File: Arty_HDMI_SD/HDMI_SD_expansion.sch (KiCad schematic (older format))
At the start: 47 parts, among them J1 0015912120, J2 1140084168, J3 0015912120, J4 2000-1-2-41-00-BK, J5 UE27AC54100, J6 0015912120, U1 TPS61232DRCT, U2 MAX3421EEHJ, Y1 KX-7_12,MHz

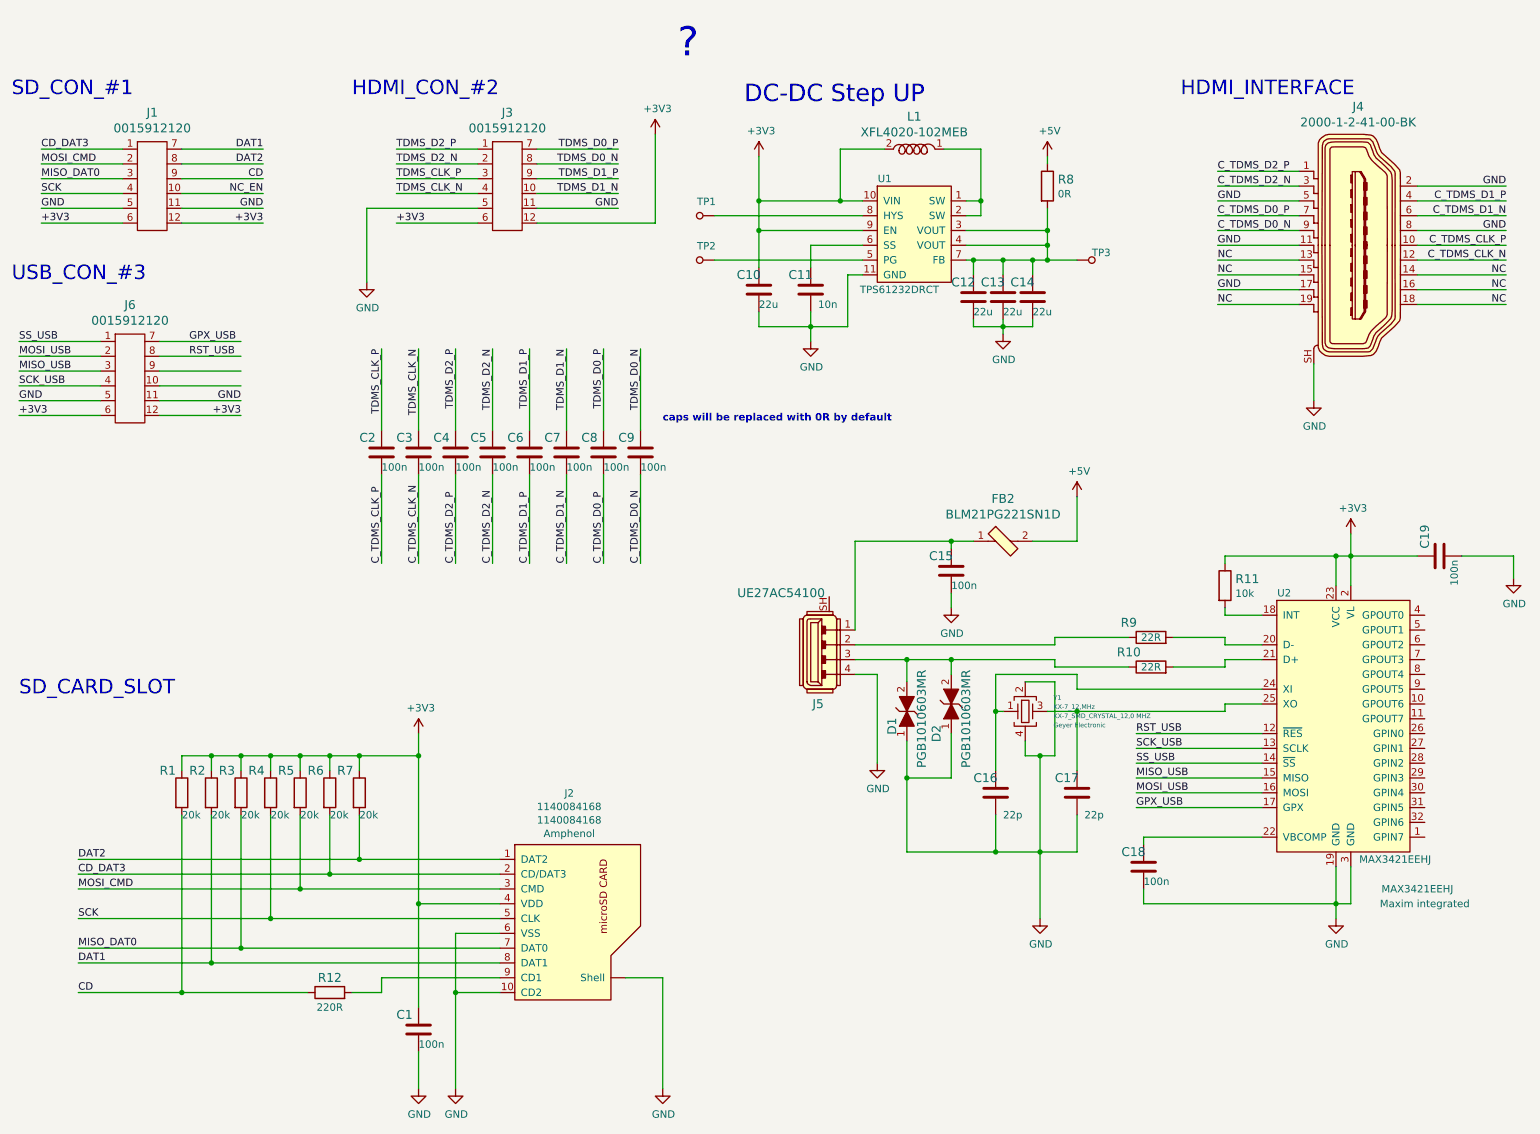
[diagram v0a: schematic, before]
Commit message: Added testpads
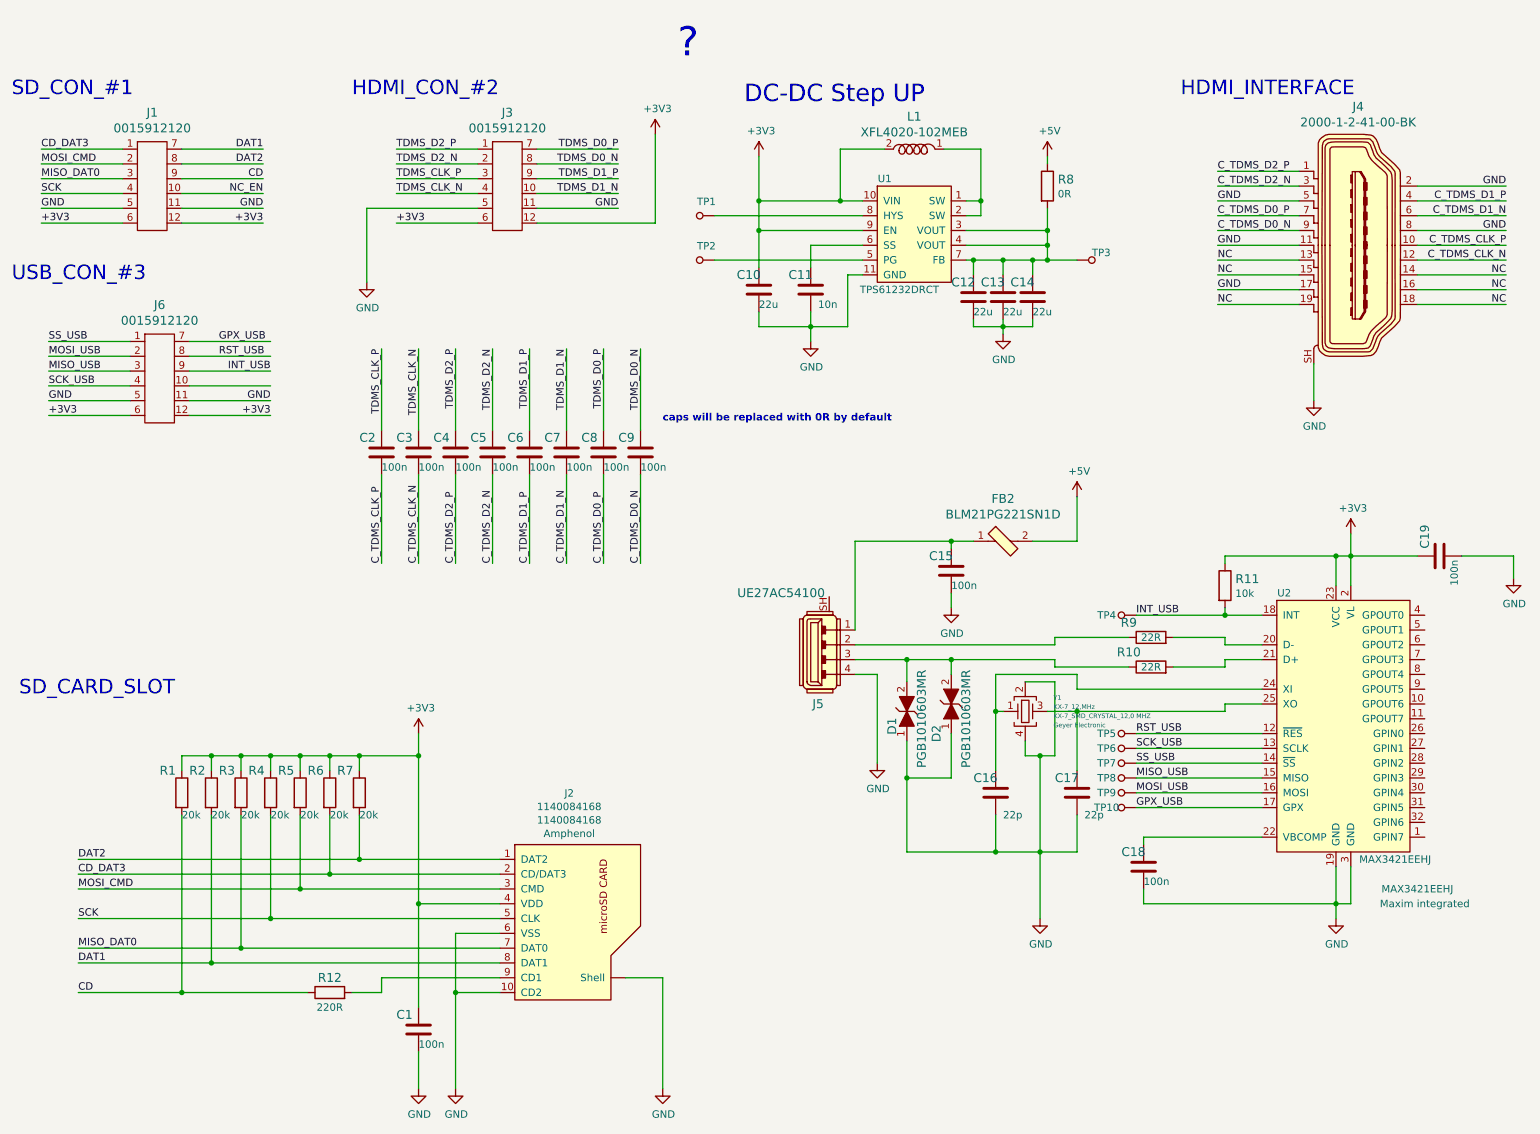
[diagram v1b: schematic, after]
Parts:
- added TP10, TP4, TP5, TP6, TP7, TP8, TP9: TP_SMD1MM, antmicro-footprints:Testpoint_smd_1mm, symbol antmicro_Test_Points:TP_SMD1MM
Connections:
- net GPX_USB: now also TP10.1
- net MISO_USB: now also TP8.1
- net MOSI_USB: now also TP9.1
- net RST_USB: now also TP5.1
- net SCK_USB: now also TP6.1
- net SS_USB: now also TP7.1
- net INT_USB: now reaches R11.2, U2.18 (INT)
- net INT_USB: now also J6.9, TP4.1
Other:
- moved on the sheet: J6
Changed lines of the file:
@@
 L antmicro_Rectangular_Connectors_Headers_Male_Pins:0015912120 J6
 U 1 1 5DC8649C
-P 1400 2600
-F 0 "J6" H 1400 3047 60  0000 C CNN
-F 1 "0015912120" H 1400 2941 60  0000 C CNN
-F 2 "antmicro-footprints:PinHeader_6x2_P2.54mm_Horizontal_Mirrored" H 1600 2800 60  0001 L CNN
-F 3 "https://www.molex.com/pdm_docs/sd/015912120_sd.pdf" H 1600 2900 60  0001 L CNN
-F 4 "0015912120" H 1600 3100 60  0001 L CNN "MPN"
-F 5 "Molex" H 1600 3700 60  0001 L CNN "Manufacturer"
-	1    1400 2600
+P 1600 2600
+F 0 "J6" H 1600 3047 60  0000 C CNN
+F 1 "0015912120" H 1600 2941 60  0000 C CNN
+F 2 "antmicro-footprints:PinHeader_6x2_P2.54mm_Horizontal_Mirrored" H 1800 2800 60  0001 L CNN
+F 3 "https://www.molex.com/pdm_docs/sd/015912120_sd.pdf" H 1800 2900 60  0001 L CNN
+F 4 "0015912120" H 1800 3100 60  0001 L CNN "MPN"
+F 5 "Molex" H 1800 3700 60  0001 L CNN "Manufacturer"
+	1    1600 2600
 	1    0    0    -1
 $EndComp
 Wire Wire Line
-	1200 2400 650  2400
+	1400 2400 850  2400
 Wire Wire Line
-	1200 2600 650  2600
-Text Label 650  2400 0    50   ~ 0
+	1400 2600 850  2600
+Text Label 850  2400 0    50   ~ 0
 SS_USB
-Text Label 650  2600 0    50   ~ 0
+Text Label 850  2600 0    50   ~ 0
 MISO_USB
 Wire Wire Line
-	2150 2400 1600 2400
+	2350 2400 1800 2400
 Wire Wire Line
-	1600 2500 2150 2500
+	1800 2500 2350 2500
 Wire Wire Line
-	1200 2500 650  2500
+	1400 2500 850  2500
 Wire Wire Line
-	1200 2700 650  2700
-Text Label 650  2500 0    50   ~ 0
+	1400 2700 850  2700
+Text Label 850  2500 0    50   ~ 0
 MOSI_USB
-Text Label 650  2700 0    50   ~ 0
+Text Label 850  2700 0    50   ~ 0
 SCK_USB
 Wire Wire Line
-	1600 2600 2150 2600
+	1800 2600 2350 2600
 Wire Wire Line
-	2150 2700 1600 2700
+	2350 2700 1800 2700
 Wire Wire Line
-	650  2800 1200 2800
-Text Label 650  2800 0    50   ~ 0
+	850  2800 1400 2800
+Text Label 850  2800 0    50   ~ 0
 GND
-Text Label 650  2900 0    50   ~ 0
+Text Label 850  2900 0    50   ~ 0
 +3V3
 Wire Wire Line
-	1200 2900 650  2900
+	1400 2900 850  2900
 Wire Wire Line
-	2150 2800 1600 2800
-Text Label 2150 2800 2    50   ~ 0
+	2350 2800 1800 2800
+Text Label 2350 2800 2    50   ~ 0
 GND
-Text Label 2150 2900 2    50   ~ 0
+Text Label 2350 2900 2    50   ~ 0
 +3V3
 Wire Wire Line
-	1600 2900 2150 2900
+	1800 2900 2350 2900
 Text Notes 600  2000 0    98   ~ 0
 USB_CON_#3
@@
 Wire Wire Line
 	6650 5850 7250 5850
-Text Label 1800 2400 0    50   ~ 0
+Text Label 2000 2400 0    50   ~ 0
 GPX_USB
-Text Label 1800 2500 0    50   ~ 0
+Text Label 2000 2500 0    50   ~ 0
 RST_USB
 Wire Wire Line
 	6450 4650 6450 5250
+Wire Wire Line
+	8800 4250 8200 4250
+Connection ~ 8800 4250
+Text Label 8200 4250 0    50   ~ 0
+INT_USB
+Text Label 2350 2600 2    50   ~ 0
+INT_USB
+$Comp
+L antmicro_Test_Points:TP_SMD1MM TP5
+U 1 1 5D79AD74
+P 8100 5050
+F 0 "TP5" V 8100 4950 50  0000 C CNN
+F 1 "TP_SMD1MM" H 8100 4950 50  0001 C CNN
+F 2 "antmicro-footprints:Testpoint_smd_1mm" H 8300 5250 60  0001 L CNN
+F 3 "" H 8300 5350 60  0001 L CNN
+	1    8100 5050
+	0    1    1    0
+$EndComp
+$Comp
+L antmicro_Test_Points:TP_SMD1MM TP6
+U 1 1 5D79AE8D
+P 8100 5150
+F 0 "TP6" V 8100 5050 50  0000 C CNN
+F 1 "TP_SMD1MM" H 8100 5050 50  0001 C CNN
+F 2 "antmicro-footprints:Testpoint_smd_1mm" H 8300 5350 60  0001 L CNN
+F 3 "" H 8300 5450 60  0001 L CNN
+	1    8100 5150
+	0    1    1    0
+$EndComp
+$Comp
+L antmicro_Test_Points:TP_SMD1MM TP7
+U 1 1 5D79AEFF
+P 8100 5250
+F 0 "TP7" V 8100 5150 50  0000 C CNN
+F 1 "TP_SMD1MM" H 8100 5150 50  0001 C CNN
+F 2 "antmicro-footprints:Testpoint_smd_1mm" H 8300 5450 60  0001 L CNN
+F 3 "" H 8300 5550 60  0001 L CNN
+	1    8100 5250
+	0    1    1    0
+$EndComp
+$Comp
+L antmicro_Test_Points:TP_SMD1MM TP8
+U 1 1 5D79AF73
+P 8100 5350
+F 0 "TP8" V 8100 5250 50  0000 C CNN
+F 1 "TP_SMD1MM" H 8100 5250 50  0001 C CNN
+F 2 "antmicro-footprints:Testpoint_smd_1mm" H 8300 5550 60  0001 L CNN
+F 3 "" H 8300 5650 60  0001 L CNN
+	1    8100 5350
+	0    1    1    0
+$EndComp
+$Comp
+L antmicro_Test_Points:TP_SMD1MM TP9
+U 1 1 5D79AFE9
+P 8100 5450
+F 0 "TP9" V 8100 5350 50  0000 C CNN
+F 1 "TP_SMD1MM" H 8100 5350 50  0001 C CNN
+F 2 "antmicro-footprints:Testpoint_smd_1mm" H 8300 5650 60  0001 L CNN
+F 3 "" H 8300 5750 60  0001 L CNN
+	1    8100 5450
+	0    1    1    0
+$EndComp
+$Comp
+L antmicro_Test_Points:TP_SMD1MM TP10
+U 1 1 5D79B061
+P 8100 5550
+F 0 "TP10" V 8100 5450 50  0000 C CNN
+F 1 "TP_SMD1MM" H 8100 5450 50  0001 C CNN
+F 2 "antmicro-footprints:Testpoint_smd_1mm" H 8300 5750 60  0001 L CNN
+F 3 "" H 8300 5850 60  0001 L CNN
+	1    8100 5550
+	0    1    1    0
+$EndComp
+$Comp
+L antmicro_Test_Points:TP_SMD1MM TP4
+U 1 1 5D79B146
+P 8100 4250
+F 0 "TP4" V 8100 4150 50  0000 C CNN
+F 1 "TP_SMD1MM" H 8100 4150 50  0001 C CNN
+F 2 "antmicro-footprints:Testpoint_smd_1mm" H 8300 4450 60  0001 L CNN
+F 3 "" H 8300 4550 60  0001 L CNN
+	1    8100 4250
+	0    1    1    0
+$EndComp
 $EndSCHEMATC
